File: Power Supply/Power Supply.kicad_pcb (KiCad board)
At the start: 2 copper layers, 84 x 96 mm, 37 parts, among them U1 LT3086ET7, U2 LT3091ET7

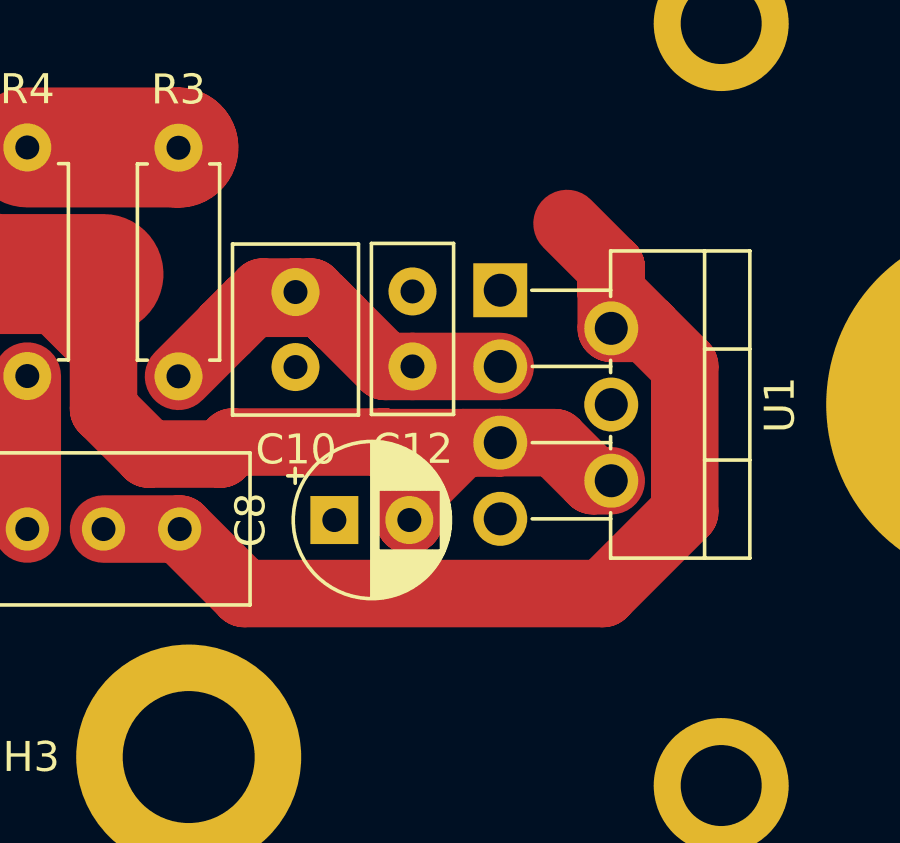
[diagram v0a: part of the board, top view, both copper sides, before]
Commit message: Fix DRC issues
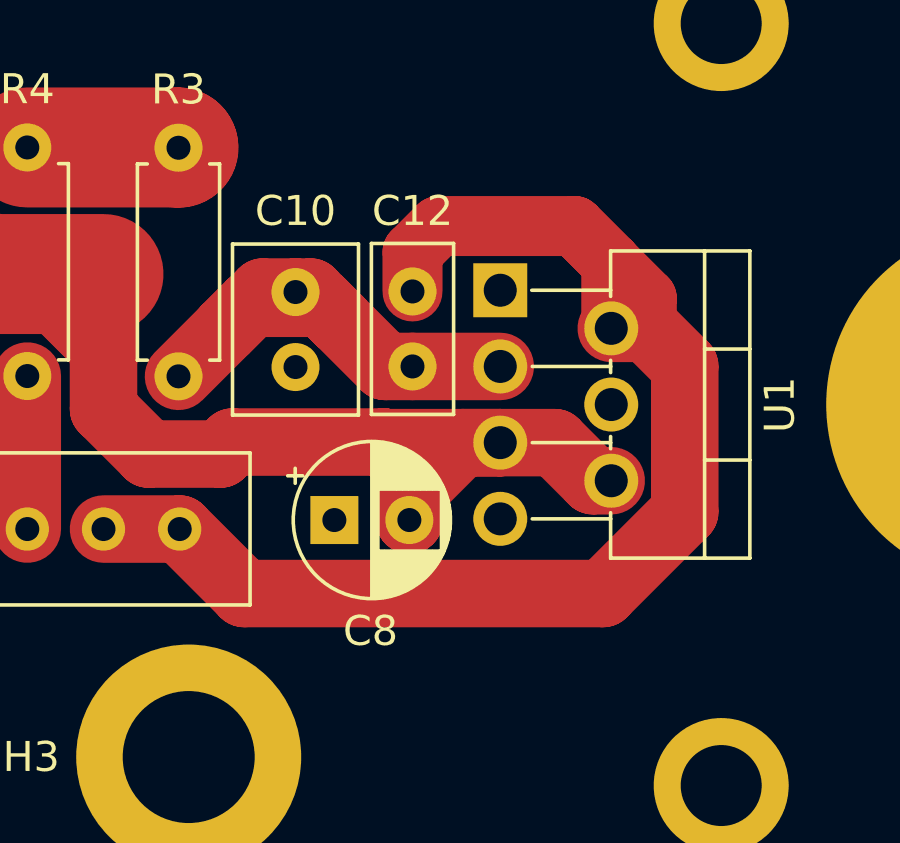
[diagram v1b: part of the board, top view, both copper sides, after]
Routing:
- net Net-(U1-SET): track 35.8 -> 44.6 mm
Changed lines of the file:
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@@
     (property "ki_description" "Mounting Hole with connection")
     (property "ki_keywords" "mounting hole")
-    (attr smd)
+    (attr through_hole)
     (fp_text reference "H5" (at 0 -5.5 unlocked) (layer "F.SilkS")
         (effects (font (size 1 1) (thickness 0.15)))
@@
     (property "ki_keywords" "cap capacitor")
     (attr through_hole)
-    (fp_text reference "C12" (at -2.75 0) (layer "F.SilkS")
+    (fp_text reference "C12" (at 5.18 0) (layer "F.SilkS")
         (effects (font (size 1 1) (thickness 0.15)))
     )
@@
     (property "ki_description" "Mounting Hole with connection")
     (property "ki_keywords" "mounting hole")
-    (attr smd)
+    (attr through_hole)
     (fp_text reference "H7" (at 7.5 0 unlocked) (layer "F.SilkS")
         (effects (font (size 1 1) (thickness 0.15)))
@@
     (property "ki_description" "Mounting Hole with connection")
     (property "ki_keywords" "mounting hole")
-    (attr smd)
+    (attr through_hole)
     (fp_text reference "H4" (at -5.25 0 unlocked) (layer "F.SilkS")
         (effects (font (size 1 1) (thickness 0.15)))
@@
     (property "ki_description" "Mounting Hole with connection")
     (property "ki_keywords" "mounting hole")
-    (attr smd)
+    (attr through_hole)
     (fp_text reference "H8" (at 0 -7 unlocked) (layer "F.SilkS")
         (effects (font (size 1 1) (thickness 0.15)))
@@
     (property "ki_keywords" "cap capacitor")
     (attr through_hole)
-    (fp_text reference "C10" (at 5.25 -0.02) (layer "F.SilkS")
+    (fp_text reference "C10" (at -2.7 0) (layer "F.SilkS")
         (effects (font (size 1 1) (thickness 0.15)))
     )
@@
     (property "ki_keywords" "cap capacitor")
     (attr through_hole)
-    (fp_text reference "C8" (at -2.794888 0 90) (layer "F.SilkS")
+    (fp_text reference "C8" (at 1.205112 3.7 180) (layer "F.SilkS")
         (effects (font (size 1 1) (thickness 0.15)))
     )
@@
     (property "ki_description" "Mounting Hole with connection")
     (property "ki_keywords" "mounting hole")
-    (attr smd)
+    (attr through_hole)
     (fp_text reference "H6" (at 0 -7 unlocked) (layer "F.SilkS")
         (effects (font (size 1 1) (thickness 0.15)))
@@
     (property "ki_description" "Mounting Hole with connection")
     (property "ki_keywords" "mounting hole")
-    (attr smd)
+    (attr through_hole)
     (fp_text reference "H3" (at -5.25 0 unlocked) (layer "F.SilkS")
         (effects (font (size 1 1) (thickness 0.15)))
@@
   (segment (start 166.45 80.05) (end 169.175 77.325) (width 2.25) (layer "F.Cu") (net 7))
   (segment (start 152.34 77.9) (end 154.49 80.05) (width 2.25) (layer "F.Cu") (net 7))
-  (segment (start 166.725 71.21) (end 166.725 69.19) (width 2.25) (layer "F.Cu") (net 7))
-  (segment (start 166.725 70.025) (end 167.91 71.21) (width 2.25) (layer "F.Cu") (net 7))
+  (segment (start 166.725 69.025) (end 166.725 71.21) (width 2) (layer "F.Cu") (net 7))
+  (segment (start 167.91 70.21) (end 167.91 71.21) (width 2) (layer "F.Cu") (net 7))
   (segment (start 167.91 71.21) (end 166.725 71.21) (width 2.25) (layer "F.Cu") (net 7))
   (segment (start 154.49 80.05) (end 166.45 80.05) (width 2.25) (layer "F.Cu") (net 7))
-  (segment (start 166.725 69.19) (end 165.25 67.715) (width 2.25) (layer "F.Cu") (net 7))
+  (segment (start 160.965 67.8) (end 165.5 67.8) (width 2) (layer "F.Cu") (net 7))
+  (segment (start 160.1 69.98) (end 160.1 68.665) (width 2) (layer "F.Cu") (net 7))
   (segment (start 149.8 77.9) (end 152.34 77.9) (width 2.25) (layer "F.Cu") (net 7))
   (segment (start 169.175 72.475) (end 167.91 71.21) (width 2.25) (layer "F.Cu") (net 7))
-  (segment (start 166.725 69.19) (end 166.725 70.025) (width 2.25) (layer "F.Cu") (net 7))
+  (segment (start 165.5 67.8) (end 166.725 69.025) (width 2) (layer "F.Cu") (net 7))
   (segment (start 169.175 77.325) (end 169.175 72.475) (width 2.25) (layer "F.Cu") (net 7))
+  (segment (start 165.5 67.8) (end 167.91 70.21) (width 2) (layer "F.Cu") (net 7))
+  (segment (start 160.1 68.665) (end 160.965 67.8) (width 2) (layer "F.Cu") (net 7))
   (segment (start 125.25 138.58) (end 125.25 138.69) (width 4) (layer "F.Cu") (net 8))
   (segment (start 125.25 138.58) (end 130.5 138.58) (width 4) (layer "F.Cu") (net 8))
